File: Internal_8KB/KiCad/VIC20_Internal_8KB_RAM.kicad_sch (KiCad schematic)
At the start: 9 parts, among them J1 UD4, J2 UE4, J3 SW, J4 Signals, U1 6264, U2 GAL16V8

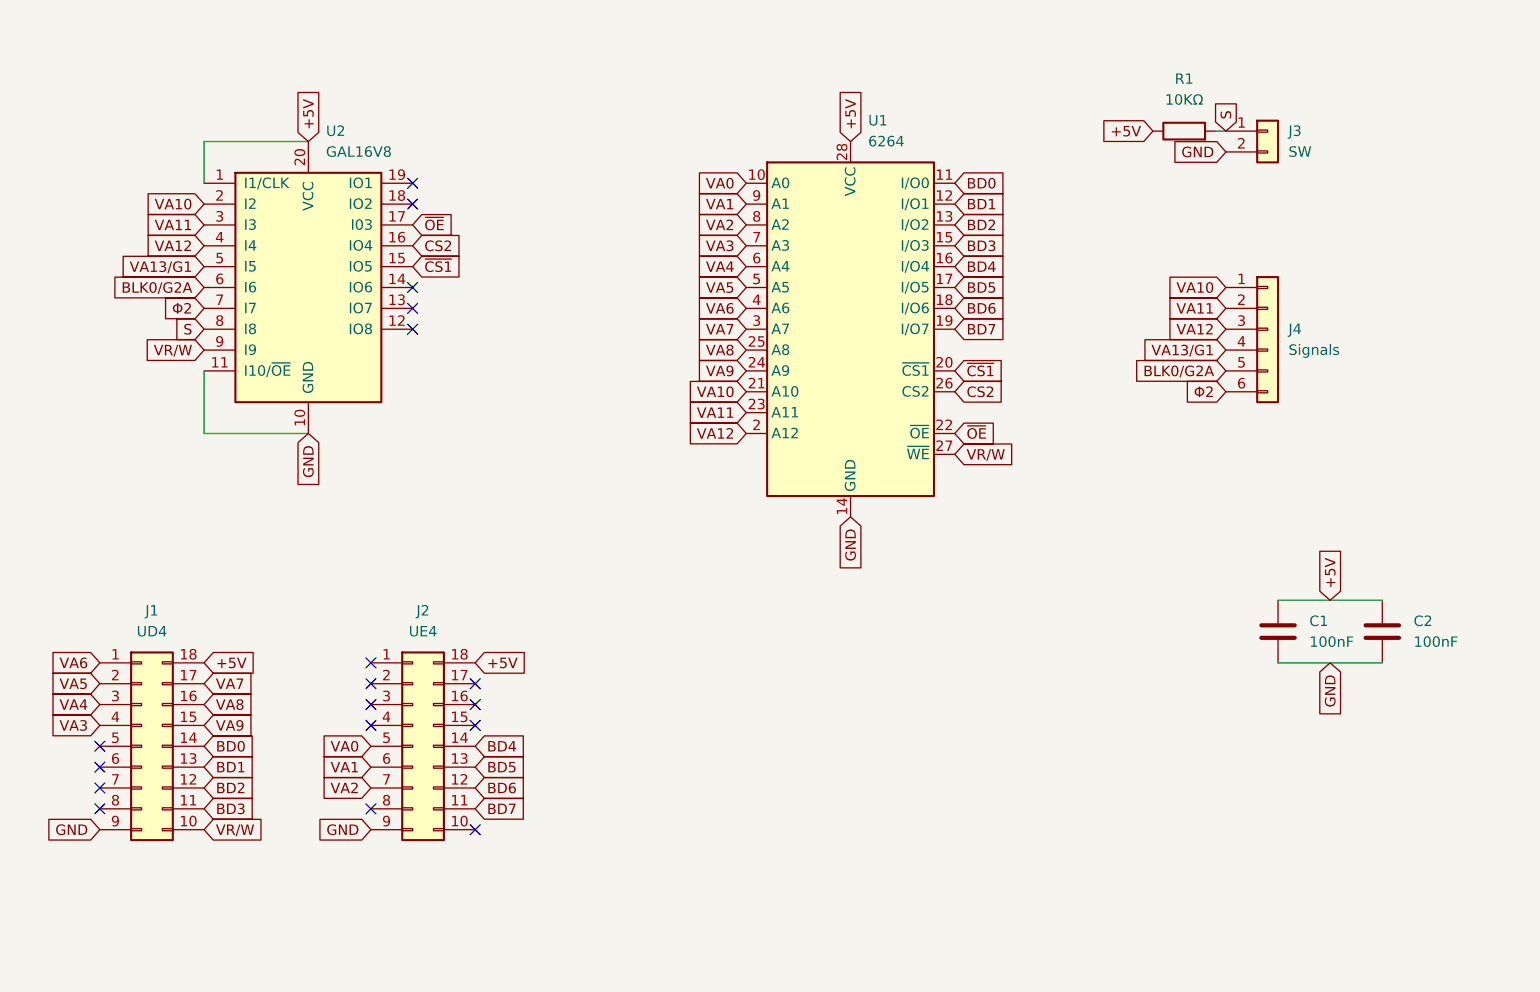
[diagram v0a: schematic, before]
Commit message: Cosmetic updates to schematic
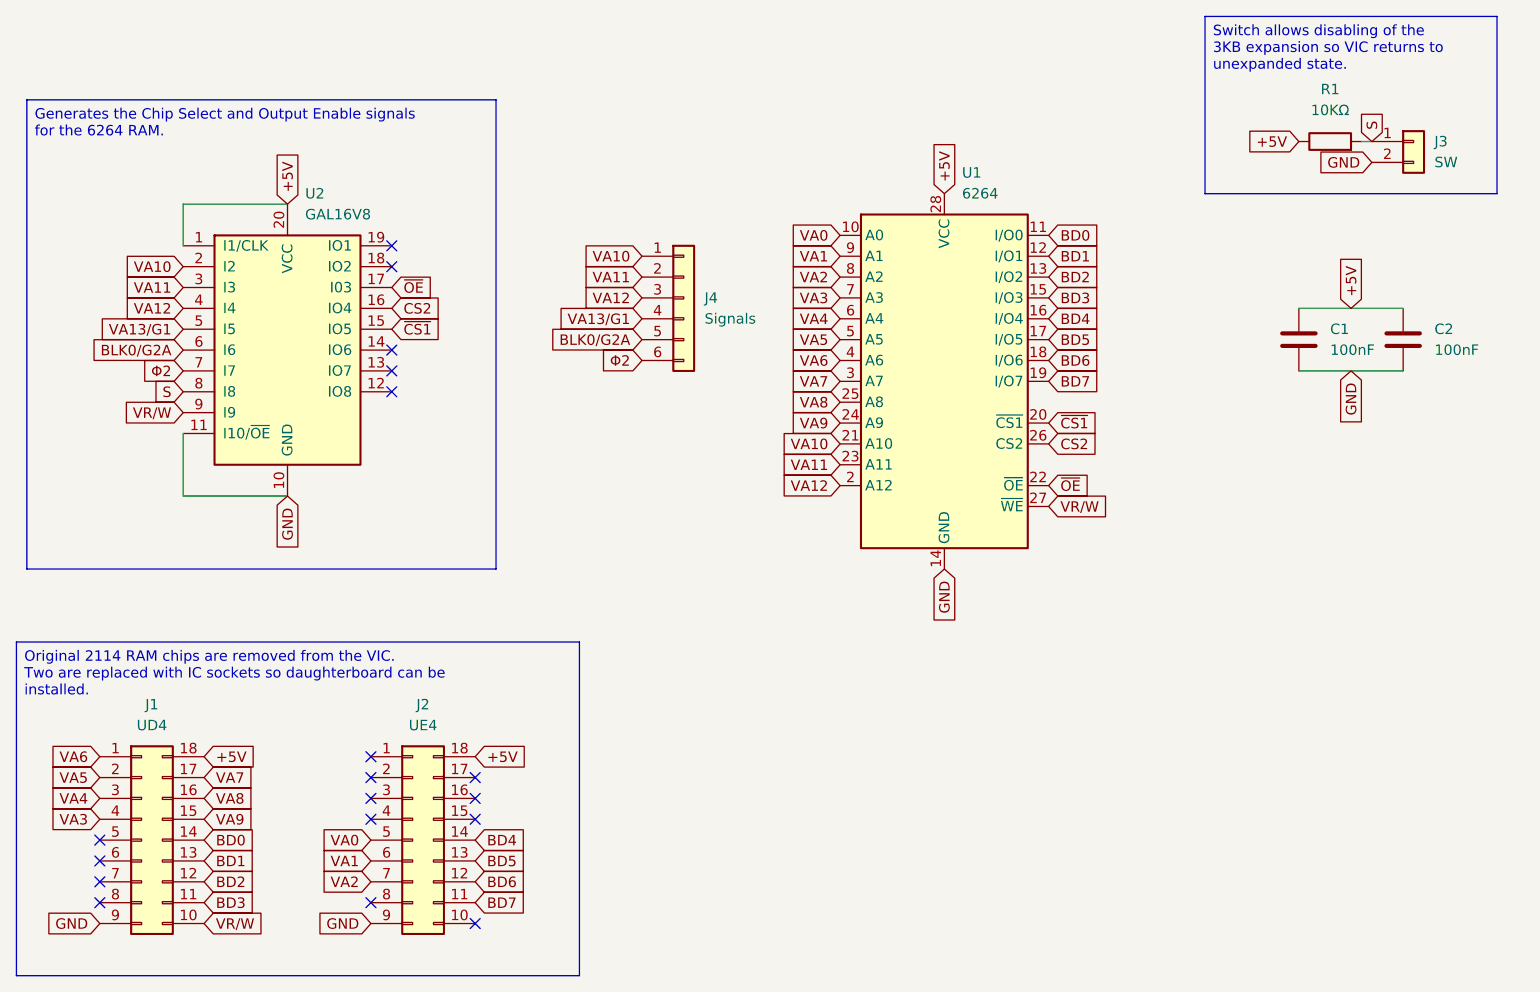
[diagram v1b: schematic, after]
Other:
- company: (none) -> Brett Hallen
- title: (none) -> Commodore VIC-20 BLK0 RAM Expansion 
- moved on the sheet: C1, C2, J1, J2, J3, J4, R1, U1, U2
